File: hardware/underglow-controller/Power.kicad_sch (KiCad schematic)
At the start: 11 parts, among them U6 BD33C0AWFP-CE2

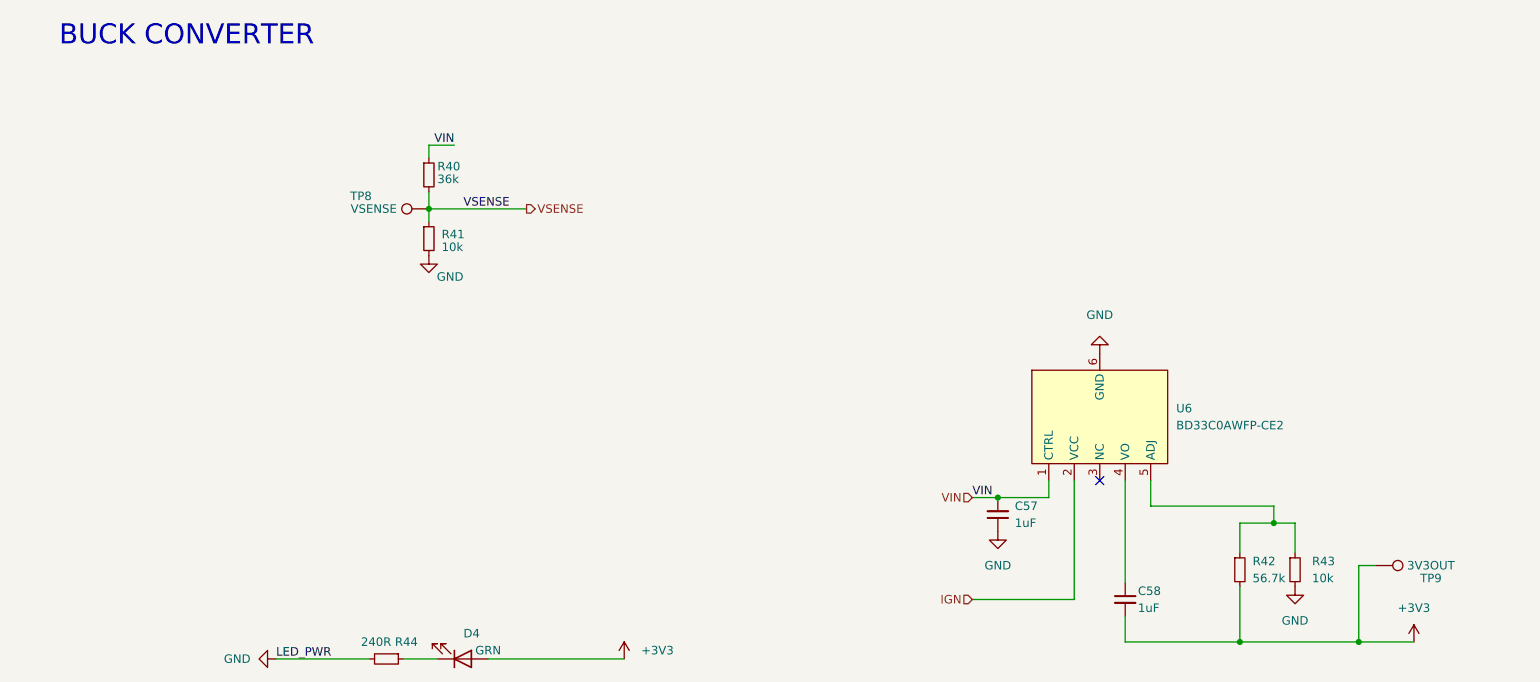
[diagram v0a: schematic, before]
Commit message: schematic almost done
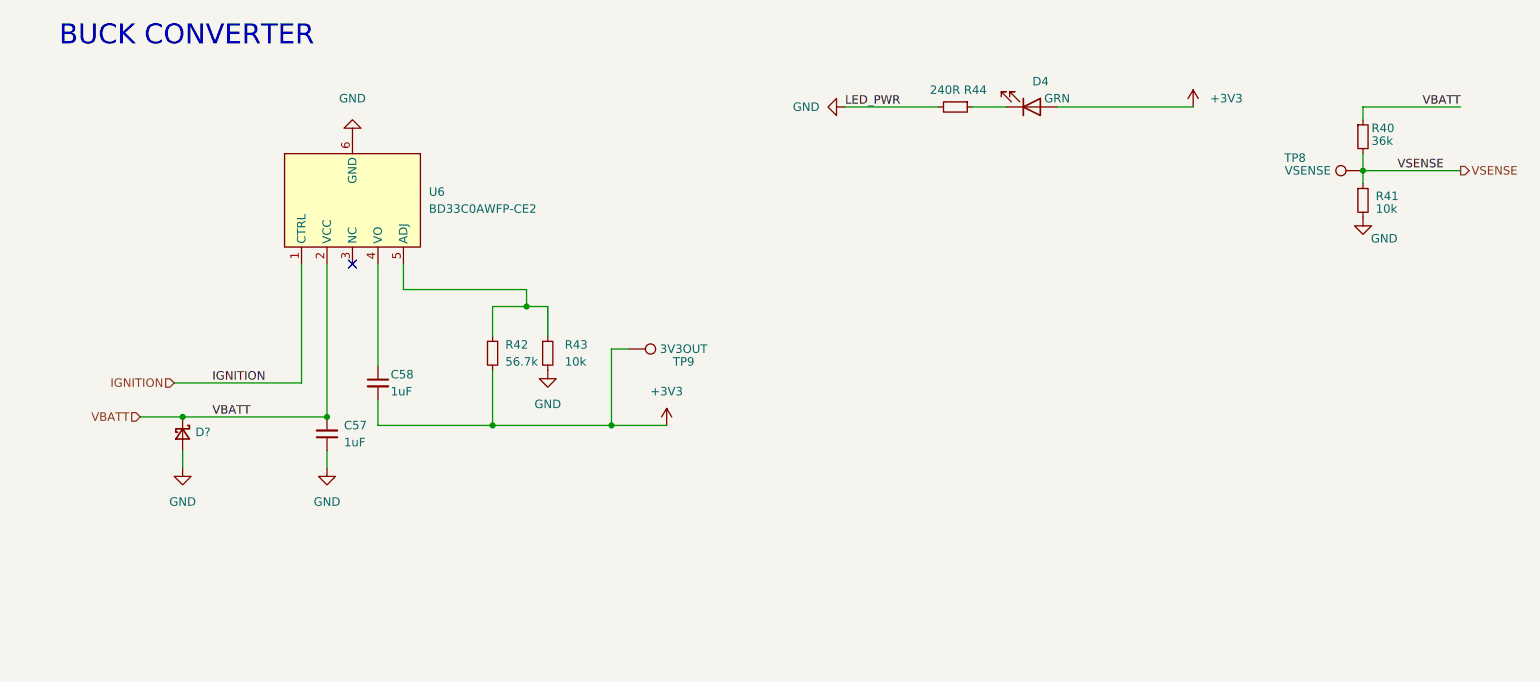
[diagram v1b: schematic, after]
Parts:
- added D?: D_Schottky_Small, Diode_SMD:D_SMA, symbol Device:D_Schottky_Small
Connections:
- net GND: now also D?.2 (A)
- net IGN renamed VBATT
- net VBATT: now also C57.2, R40.1, D?.1 (K)
- removed net VIN: C57.2, R40.1, U6.1 (CTRL)
- new net IGNITION: U6.1 (CTRL)
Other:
- moved on the sheet: C57, C58, D4, R40, R41, R42, R43, R44, TP8, TP9, U6
